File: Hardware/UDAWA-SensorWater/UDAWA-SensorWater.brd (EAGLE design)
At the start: 160 x 100 mm, 9 parts

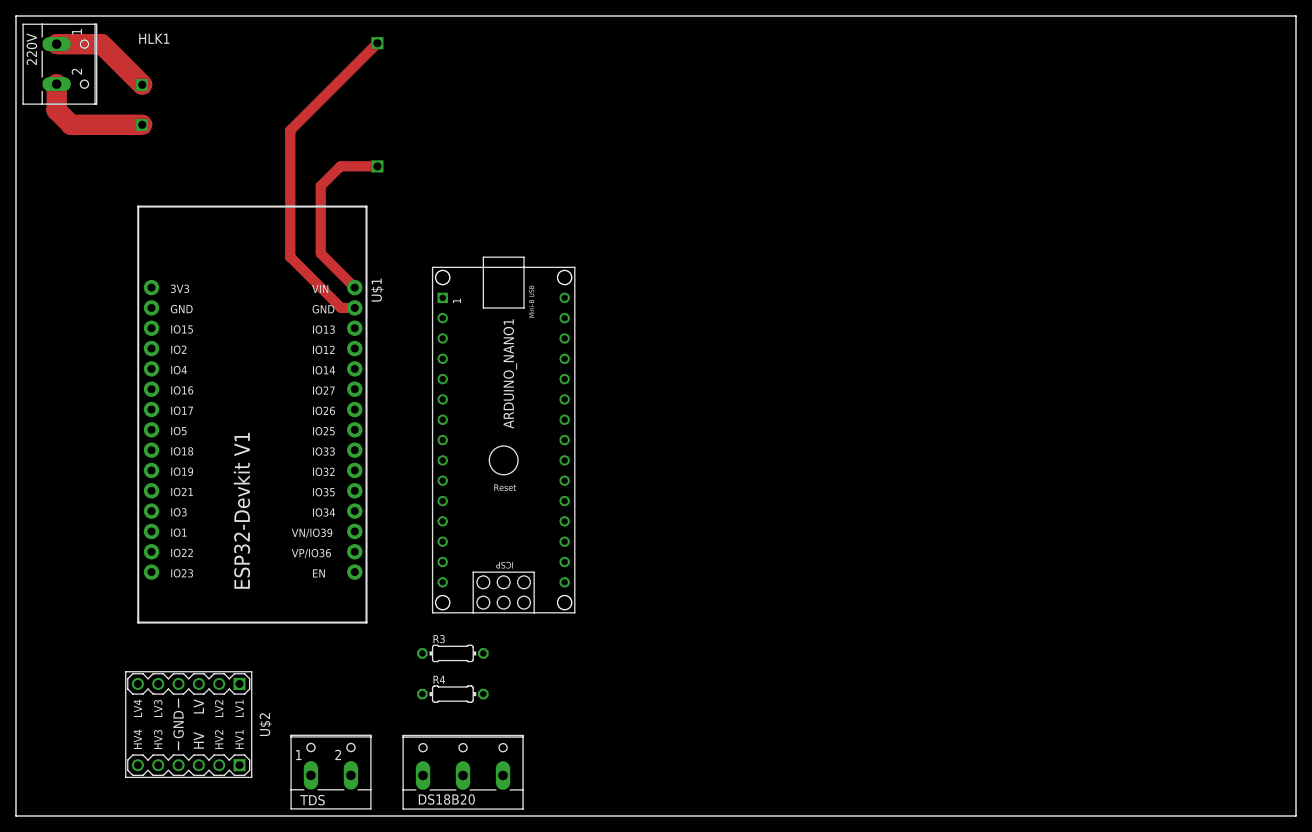
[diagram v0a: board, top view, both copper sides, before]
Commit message: Routing PCB #6
Routing PCB
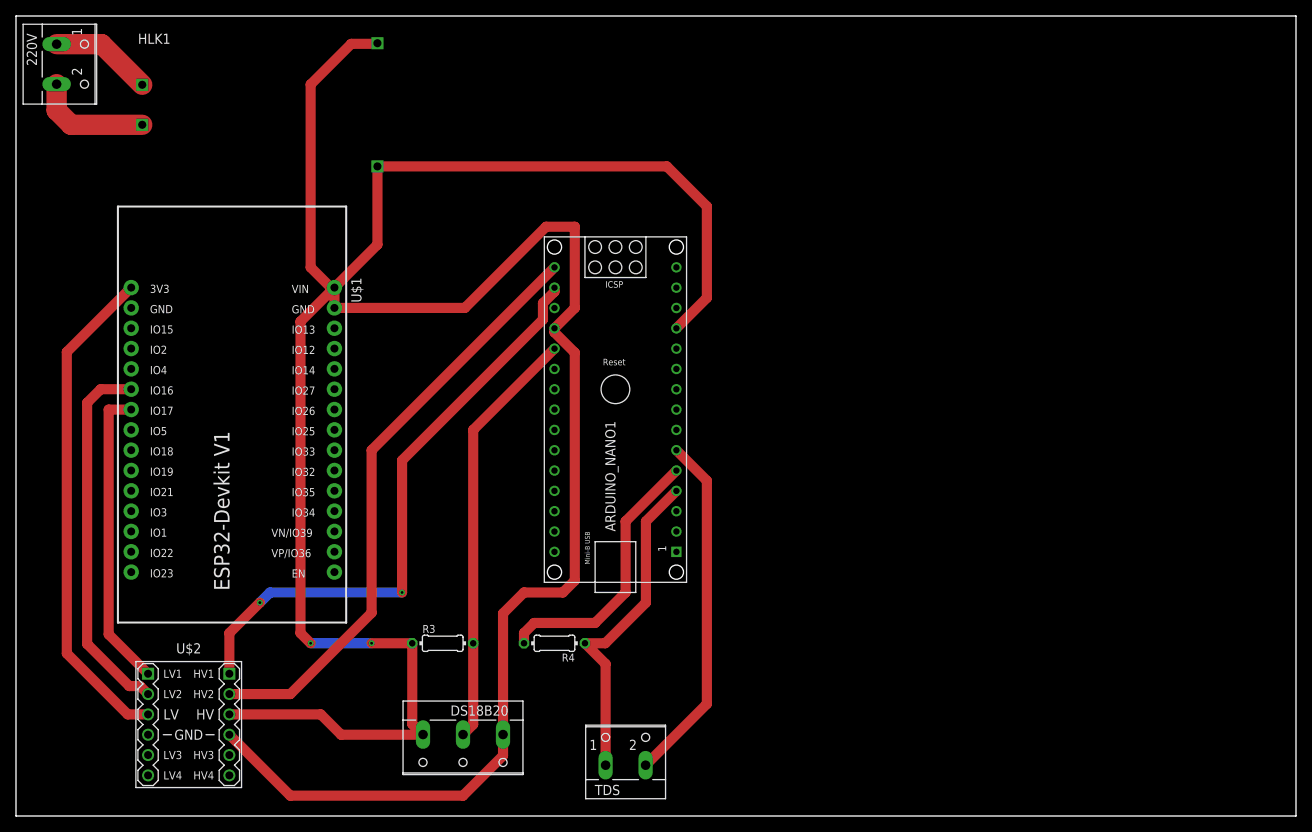
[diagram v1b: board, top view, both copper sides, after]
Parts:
- moved TDS 36.9 mm to (76.2, 7.62)
- moved ARDUINO_NANO1 16.6 mm to (74.9, 53.3), turned to 90 degrees
- moved R4 14.2 mm to (67.3, 21.6), turned to 180 degrees
- moved DS18B20 2.54 mm to (55.9, 8.89), turned to 180 degrees
- moved U$1 2.54 mm to (26.7, 49.5)
- moved R3 1.80 mm to (53.3, 21.6)
- turned U$2 to 0 degrees
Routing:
- net 5V: track 22.5 -> 174.1 mm, vias 0 -> 2
- net GND: track 41.9 -> 188.1 mm
- net HV1: track 0.00 -> 74.8 mm, vias 0 -> 2
- net HV2: track 0.00 -> 74.6 mm
- net 3V3: track 0.00 -> 62.4 mm
- net D2: track 0.00 -> 53.0 mm
- net LV2: track 0.00 -> 46.6 mm
- net A2: track 0.00 -> 44.1 mm
- net A0: track 0.00 -> 41.6 mm
- net LV1: track 0.00 -> 37.9 mm
- net A1: track 0.00 -> 33.9 mm
